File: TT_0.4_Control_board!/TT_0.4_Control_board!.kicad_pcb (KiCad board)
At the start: 2 copper layers, 150 x 90 mm, 1 part

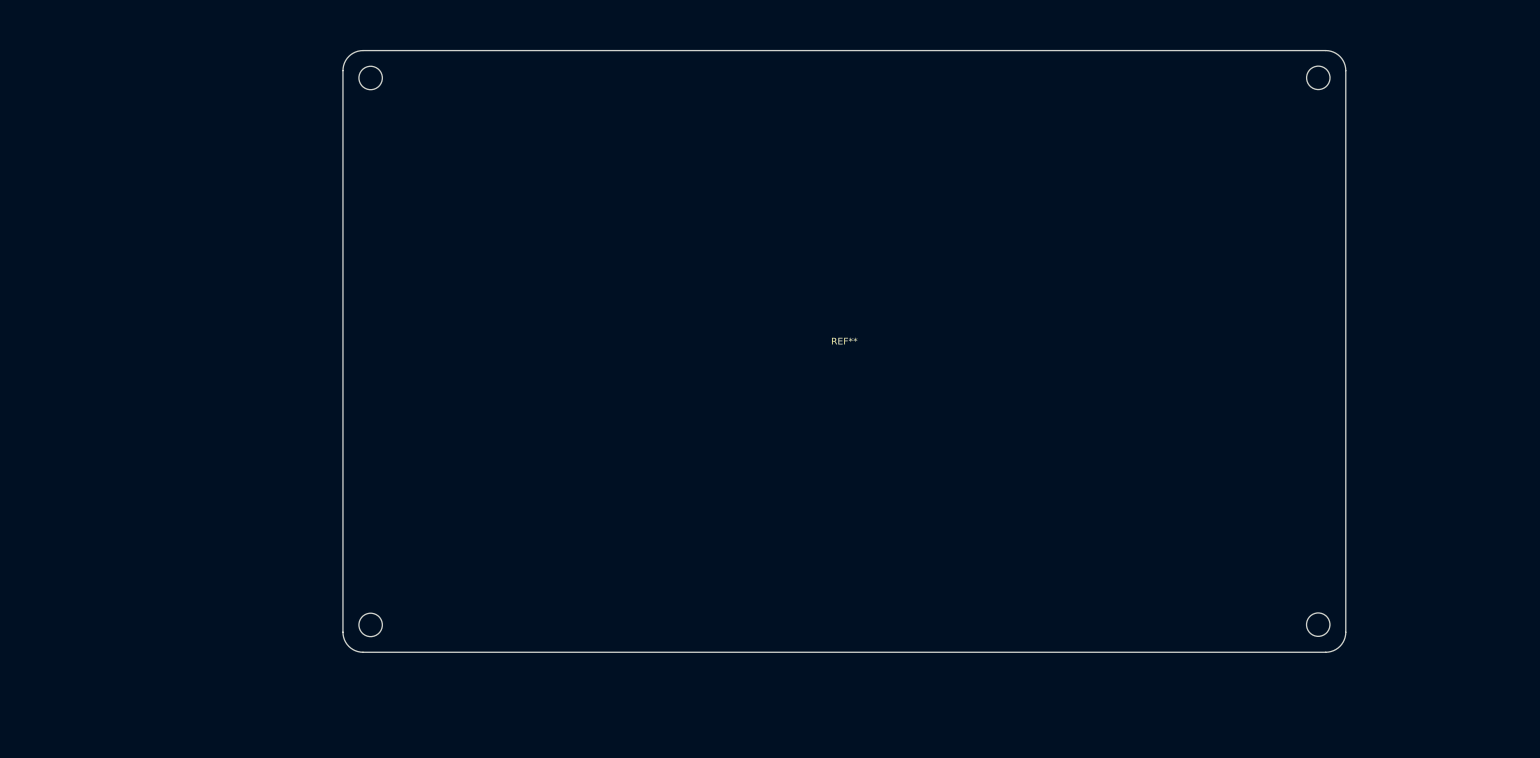
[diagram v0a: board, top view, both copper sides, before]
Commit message: Final_PCB_Design
This push final, updated push TT-0.4:Controller
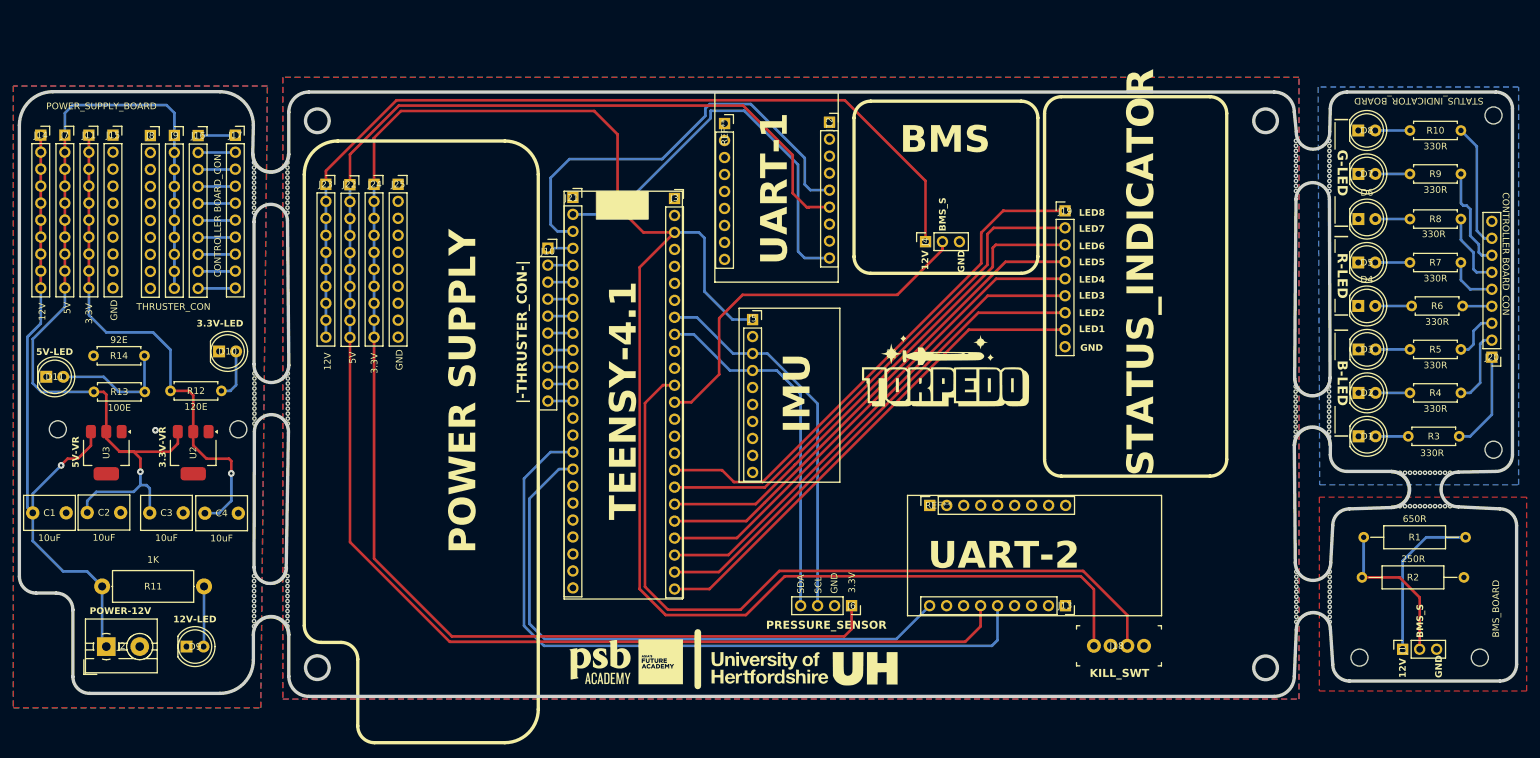
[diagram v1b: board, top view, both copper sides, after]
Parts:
- removed the REF** at (156.0, 97.0)
- added C1: 10uF, Capacitor_THT:C_Disc_D7.5mm_W5.0mm_P5.00mm, F.Cu at (34.6, 122.2)
- added C2: 10uF, Capacitor_THT:C_Disc_D7.5mm_W5.0mm_P5.00mm, F.Cu at (42.8, 122.1)
- added C3: 10uF, Capacitor_THT:C_Disc_D7.5mm_W5.0mm_P5.00mm, F.Cu at (52.1, 122.2)
- added C4: 10uF, Capacitor_THT:C_Disc_D7.5mm_W5.0mm_P5.00mm, F.Cu at (60.4, 122.2)
- added D1: B_LED, LED_THT:LED_D5.0mm, F.Cu at (232.9, 110.7)
- added D10: Green_POW_LED_3.3V, LED_THT:LED_D5.0mm, F.Cu at (62.5, 98.0)
- added D11: Green_POW_LED_5V, LED_THT:LED_D5.0mm, F.Cu at (36.6, 101.8)
- added D2: B_LED, LED_THT:LED_D5.0mm, F.Cu at (232.9, 104.2)
- added D3: B_LED, LED_THT:LED_D5.0mm, F.Cu at (232.9, 97.7)
- added D4: R_LED, LED_THT:LED_D5.0mm, F.Cu at (232.9, 91.2)
- added D5: R_LED, LED_THT:LED_D5.0mm, F.Cu at (232.9, 84.7)
- added D6: G_LED, LED_THT:LED_D5.0mm, F.Cu at (232.9, 78.2)
- added D7: G_LED, LED_THT:LED_D5.0mm, F.Cu at (232.9, 71.5)
- added D8: G_LED, LED_THT:LED_D5.0mm, F.Cu at (232.9, 65.0)
- added D9: RED_POW_LED, LED_THT:LED_D5.0mm, F.Cu at (57.6, 142.2)
- added J1: Conn_01x03_Socket, Connector_PinSocket_2.54mm:PinSocket_1x03_P2.54mm_Vertical, F.Cu at (239.5, 142.6)
- added J10: Conn_01x10_Socket_Thruster_Teensy_pins, Connector_PinSocket_2.54mm:PinSocket_1x10_P2.54mm_Vertical, F.Cu at (111.7, 82.6)
- added J11: Conn_01x10_Socket_3.3V, Connector_PinSocket_2.54mm:PinSocket_1x10_P2.54mm_Vertical, F.Cu at (43.0, 65.7)
- added J12: Conn_01x09_Socket_TR, Connector_PinSocket_2.54mm:PinSocket_1x09_P2.54mm_Vertical, F.Cu at (153.8, 63.7)
- added J13: Conn_01x09_Socket_TR, Connector_PinSocket_2.54mm:PinSocket_1x09_P2.54mm_Vertical, F.Cu at (189.1, 136.0)
- added J14: Conn_01x10_Socket_12V, Connector_PinSocket_2.54mm:PinSocket_1x10_P2.54mm_Vertical, F.Cu at (35.8, 65.7)
- added J15: Conn_01x10_Socket_GND, Connector_PinSocket_2.54mm:PinSocket_1x10_P2.54mm_Vertical, F.Cu at (46.6, 65.7)
- added J16: Conn_01x10_Socket_Thruster_C_pins, Connector_PinSocket_2.54mm:PinSocket_1x10_P2.54mm_Vertical, F.Cu at (59.3, 65.7)
- added J17: Conn_01x10_Socket_Thruster_C_pins, Connector_PinSocket_2.54mm:PinSocket_1x10_P2.54mm_Vertical, F.Cu at (64.9, 65.7)
- added J18: JST_S_Kill, digikey-footprints:PinHeader_1x4_P2.5mm_Drill1.1mm, F.Cu at (193.3, 142.0)
- added J19: Conn_01x09_Socket, Connector_PinHeader_2.54mm:PinHeader_1x09_P2.54mm_Vertical, F.Cu at (189.0, 77.0)
- added J2: Pow_Conn, TerminalBlock:TerminalBlock_MaiXu_MX126-5.0-02P_1x02_P5.00mm, F.Cu at (45.6, 142.2)
- added J20: Conn_01x09_Socket, Connector_PinHeader_2.54mm:PinHeader_1x09_P2.54mm_Vertical, F.Cu at (252.8, 98.9)
- added J21: Conn_01x24_Socket_TL, Connector_PinSocket_2.54mm:PinSocket_1x24_P2.54mm_Vertical, F.Cu at (115.4, 75.0)
- added J22: Conn_01x10_Socket-5V, Connector_PinSocket_2.54mm:PinSocket_1x10_P2.54mm_Vertical, F.Cu at (82.0, 73.1)
- added J23: Conn_01x10_Socket_12V, Connector_PinSocket_2.54mm:PinSocket_1x10_P2.54mm_Vertical, F.Cu at (78.5, 73.0)
- added J24: Conn_01x10_Socket_3.3V, Connector_PinSocket_2.54mm:PinSocket_1x10_P2.54mm_Vertical, F.Cu at (85.7, 73.0)
- added J25: Conn_01x10_Socket_GND, Connector_PinSocket_2.54mm:PinSocket_1x10_P2.54mm_Vertical, F.Cu at (89.2, 73.0)
- added J3: Conn_01x24_Socket_TR, Connector_PinSocket_2.54mm:PinSocket_1x24_P2.54mm_Vertical, F.Cu at (130.6, 75.1)
- added J4: Conn_01x03_Socket, Connector_PinSocket_2.54mm:PinSocket_1x03_P2.54mm_Vertical, F.Cu at (168.1, 81.6)
- added J5: MPU9250, Connector_PinSocket_2.54mm:PinSocket_1x10_P2.54mm_Vertical, F.Cu at (142.3, 93.2)
- added J6: MS5837_30, Connector_PinSocket_2.54mm:PinSocket_1x04_P2.54mm_Vertical, F.Cu at (157.1, 136.0)
- added J7: Conn_01x10_Socket-5V, Connector_PinSocket_2.54mm:PinSocket_1x10_P2.54mm_Vertical, F.Cu at (39.4, 65.7)
- added J8: Conn_01x10_Socket_Thruster_GND, Connector_PinSocket_2.54mm:PinSocket_1x10_P2.54mm_Vertical, F.Cu at (52.2, 65.7)
- added J9: Conn_01x10_Socket_Thruster_5V, Connector_PinSocket_2.54mm:PinSocket_1x10_P2.54mm_Vertical, F.Cu at (55.8, 65.7)
- added R1: 650R, Resistor_THT:R_Axial_DIN0309_L9.0mm_D3.2mm_P15.24mm_Horizontal, F.Cu at (248.9, 125.8)
- added R10: 330R, Resistor_THT:R_Axial_DIN0207_L6.3mm_D2.5mm_P7.62mm_Horizontal, F.Cu at (240.6, 65.0)
- added R11: 1K, Resistor_THT:R_Axial_DIN0414_L11.9mm_D4.5mm_P15.24mm_Horizontal, F.Cu at (45.0, 133.2)
- added R12: 120E, Resistor_THT:R_Axial_DIN0207_L6.3mm_D2.5mm_P7.62mm_Horizontal, F.Cu at (55.2, 103.9)
- added R13: 100E, Resistor_THT:R_Axial_DIN0207_L6.3mm_D2.5mm_P7.62mm_Horizontal, F.Cu at (43.7, 104.0)
- added R14: 92E, Resistor_THT:R_Axial_DIN0207_L6.3mm_D2.5mm_P7.62mm_Horizontal, F.Cu at (51.3, 98.7)
- added R2: 250R, Resistor_THT:R_Axial_DIN0309_L9.0mm_D3.2mm_P15.24mm_Horizontal, F.Cu at (233.4, 131.8)
- added R3: 330R, Resistor_THT:R_Axial_DIN0207_L6.3mm_D2.5mm_P7.62mm_Horizontal, F.Cu at (240.3, 110.7)
- added R4: 330R, Resistor_THT:R_Axial_DIN0207_L6.3mm_D2.5mm_P7.62mm_Horizontal, F.Cu at (240.6, 104.2)
- added R5: 330R, Resistor_THT:R_Axial_DIN0207_L6.3mm_D2.5mm_P7.62mm_Horizontal, F.Cu at (240.6, 97.7)
- added R6: 330R, Resistor_THT:R_Axial_DIN0207_L6.3mm_D2.5mm_P7.62mm_Horizontal, F.Cu at (240.8, 91.2)
- added R7: 330R, Resistor_THT:R_Axial_DIN0207_L6.3mm_D2.5mm_P7.62mm_Horizontal, F.Cu at (240.6, 84.7)
- added R8: 330R, Resistor_THT:R_Axial_DIN0207_L6.3mm_D2.5mm_P7.62mm_Horizontal, F.Cu at (240.6, 78.2)
- added R9: 330R, Resistor_THT:R_Axial_DIN0207_L6.3mm_D2.5mm_P7.62mm_Horizontal, F.Cu at (240.6, 71.5)
- added REF**: PinSocket_1x09_P2.54mm_Vertical, Connector_PinSocket_2.54mm:PinSocket_1x09_P2.54mm_Vertical, F.Cu at (138.1, 63.9)
- added REF**: PSB Logo, AUV_Custom_design:PSB Logo, F.Cu at (123.1, 145.0)
- added REF**: PinSocket_1x09_P2.54mm_Vertical, Connector_PinSocket_2.54mm:PinSocket_1x09_P2.54mm_Vertical, F.Cu at (168.8, 121.0)
- added REF**: Team Torpedo Logo, AUV_Custom_design:Team Torpedo Logo, F.Cu at (171.1, 102.0)
- added REF**: UH_Logo, AUV_Custom_design:UH_Logo, F.Cu at (149.1, 145.4)
- added U2: LM1117T-3.3, Package_TO_SOT_SMD:SOT-223-3_TabPin2, F.Cu at (58.6, 113.2)
- added U3: LM1117T-5V, Package_TO_SOT_SMD:SOT-223-3_TabPin2, F.Cu at (45.6, 113.2)
- added mouse-bite-5mm-slot: VAL**, Panelization.pretty-master:mouse-bite-5mm-slot, F.Cu at (226.1, 134.7)
- added mouse-bite-5mm-slot: VAL**, Panelization.pretty-master:mouse-bite-5mm-slot, F.Cu at (70.2, 135.3)
- added mouse-bite-5mm-slot: VAL**, Panelization.pretty-master:mouse-bite-5mm-slot, F.Cu at (242.8, 118.7)
- added mouse-bite-5mm-slot: VAL**, Panelization.pretty-master:mouse-bite-5mm-slot, F.Cu at (70.2, 73.5)
- added mouse-bite-5mm-slot: VAL**, Panelization.pretty-master:mouse-bite-5mm-slot, F.Cu at (70.2, 105.0)
- added mouse-bite-5mm-slot: VAL**, Panelization.pretty-master:mouse-bite-5mm-slot, F.Cu at (226.0, 107.0)
- added mouse-bite-5mm-slot: VAL**, Panelization.pretty-master:mouse-bite-5mm-slot, F.Cu at (226.1, 70.2)
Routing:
- net 3.3V: track 0.00 -> 362.1 mm
- net 5V: track 0.00 -> 246.9 mm
- net P_5V: track 0.00 -> 141.5 mm, vias 0 -> 1
- net 12V: track 0.00 -> 133.2 mm
- net S_KILL: track 0.00 -> 116.3 mm
- net RX2: track 0.00 -> 108.6 mm
- net P_12V: track 0.00 -> 101.0 mm, vias 0 -> 1
- net TX2: track 0.00 -> 89.9 mm
- net LED8: track 0.00 -> 78.7 mm
- net LED7: track 0.00 -> 77.2 mm
- net LED6: track 0.00 -> 76.2 mm
- net P_3.3V: track 0.00 -> 75.9 mm, vias 0 -> 1
- net LED4: track 0.00 -> 74.5 mm
- net LED3: track 0.00 -> 74.5 mm
- net LED2: track 0.00 -> 74.5 mm
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- added copper zone on F.Cu, net BMS_GND
- added copper zone on B.Cu, net GND
- added copper zone on F.Cu, net GND
- added copper zone on B.Cu, net L_GND
- added copper zone on B.Cu, net P_GND
- added copper zone on F.Cu, net P_GND
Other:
- board size 150 x 90 mm -> 224 x 90.4 mm
- board text added: "12V"
- board text added: "12V-LED"
- board text added: "3.3V"
- board text added: "3.3V-LED"
- board text added: "3.3V-VR"
- board text added: "5V"
- board text added: "5V-LED"
- board text added: "5V-VR"
- board text added: "BMS"
- board text added: "BMS_BOARD"
- board text added: "BMS_S"
- board text added: "CONTROLLER BOARD_CON"
- board text added: "GND"
- board text added: "IMU"
- board text added: "KILL_SWT"
- board text added: "LED1"
- board text added: "LED2"
- board text added: "LED3"
- board text added: "LED4"
- board text added: "LED5"
- board text added: "LED6"
- board text added: "LED7"
- board text added: "LED8"
- board text added: "POWER SUPPLY"
- board text added: "POWER-12V"
- board text added: "POWER_SUPPLY_BOARD"
- board text added: "PRESSURE_SENSOR"
- board text added: "SCL"
- board text added: "SDA"
- board text added: "STATUS_INDICATOR"
- board text added: "STATUS_INDICATOR_BOARD"
- board text added: "TEENSY-4.1"
- board text added: "THRUSTER_CON"
- board text added: "UART-1"
- board text added: "UART-2"
- board text added: "|-THRUSTER_CON-|"
- board text added: "|__R-LED__|"
- board text added: "|____B-LED____|"
- board text added: "|____G-LED____|"
